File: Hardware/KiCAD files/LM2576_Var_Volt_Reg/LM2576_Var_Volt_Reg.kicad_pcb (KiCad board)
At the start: 2 copper layers, 48 x 48 mm, 14 parts, among them J1 Conn_01x03_Pin, U2 LM2576HVS-ADJ

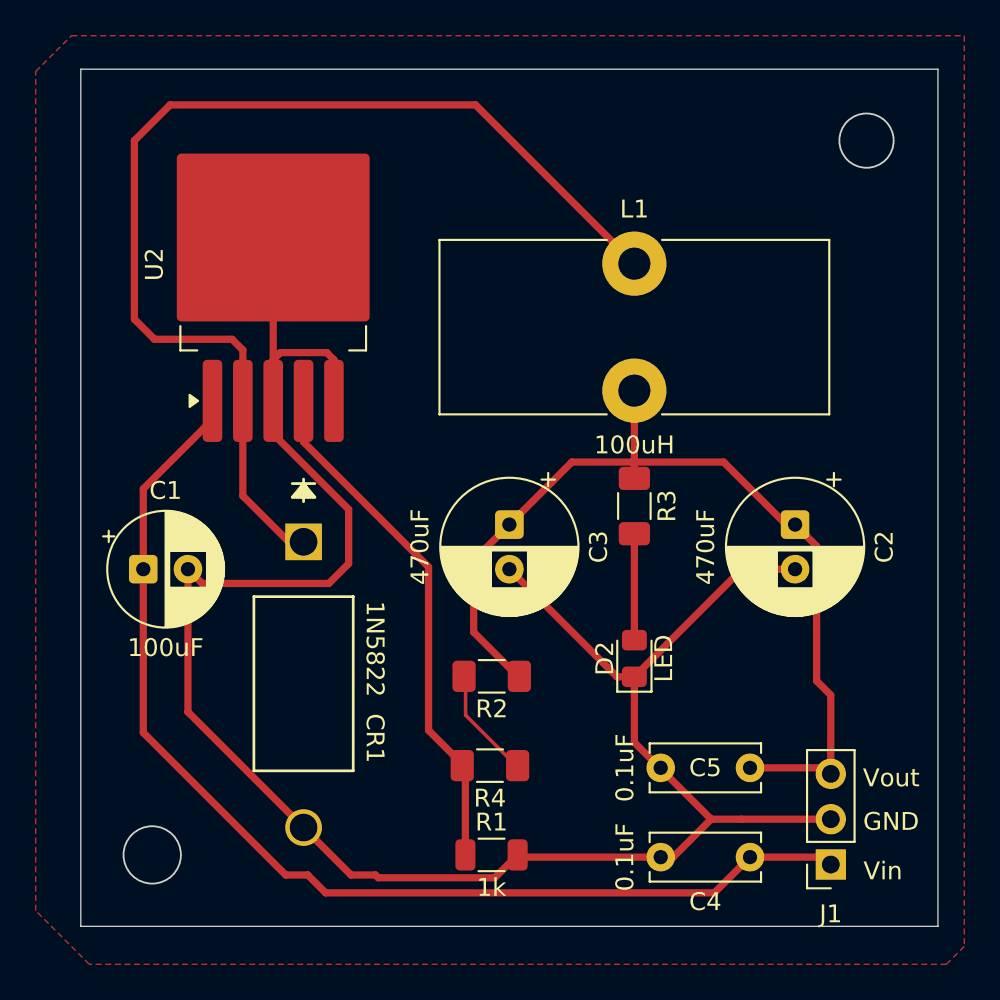
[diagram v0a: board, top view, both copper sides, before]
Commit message: general update stuff
- updated PCBs
- removed marlin submodule
- played with firmware
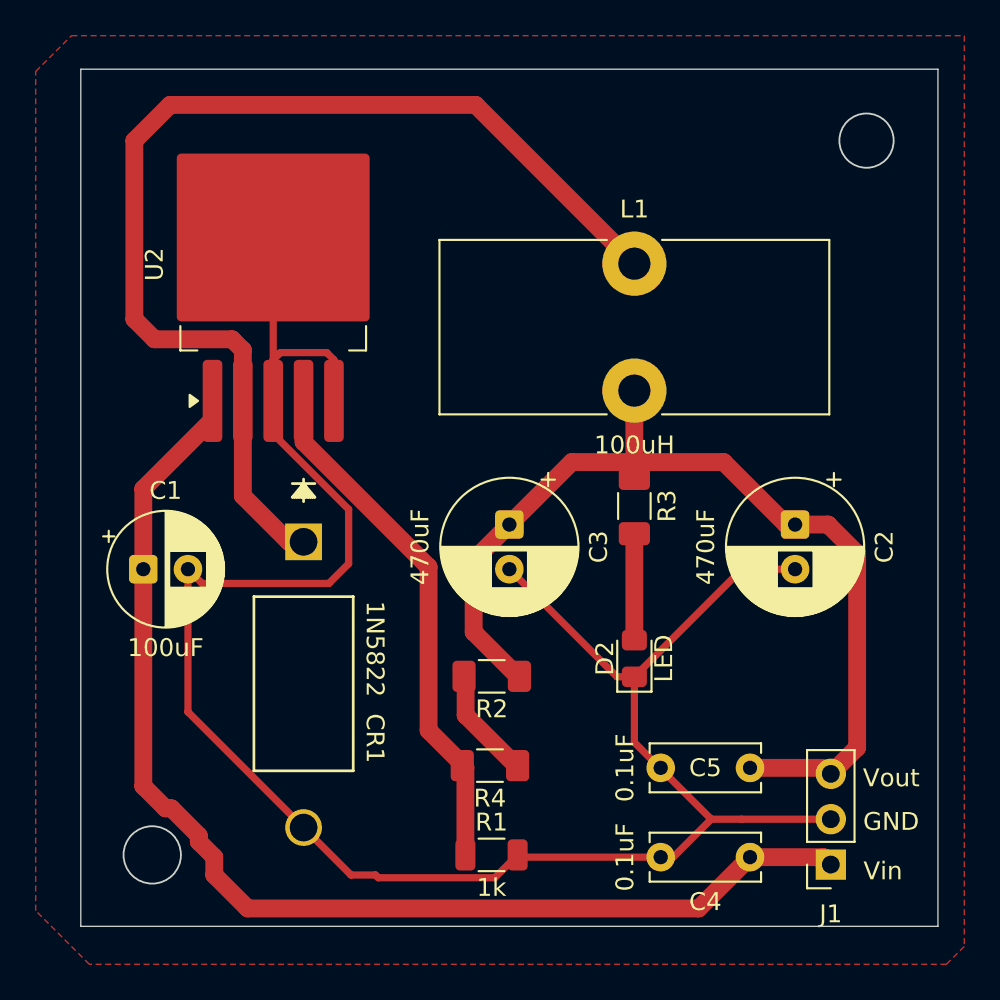
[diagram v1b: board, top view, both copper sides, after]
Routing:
- net /Vin: track 63.4 -> 66.7 mm
- net /Vout: track 53.7 -> 56.0 mm
